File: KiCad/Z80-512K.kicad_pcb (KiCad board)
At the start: 2 copper layers, 99.1 x 49.9 mm, 32 parts, among them J1 VBAT, J2 JTAG, J3 RC2014_BUS, J4 RC2014_EXT, U1 Z84C00, U2 SST39SF040, U3 AS6C4008, U4 ATF1504AS, U5 ADM693A, X1 7.3728MHz

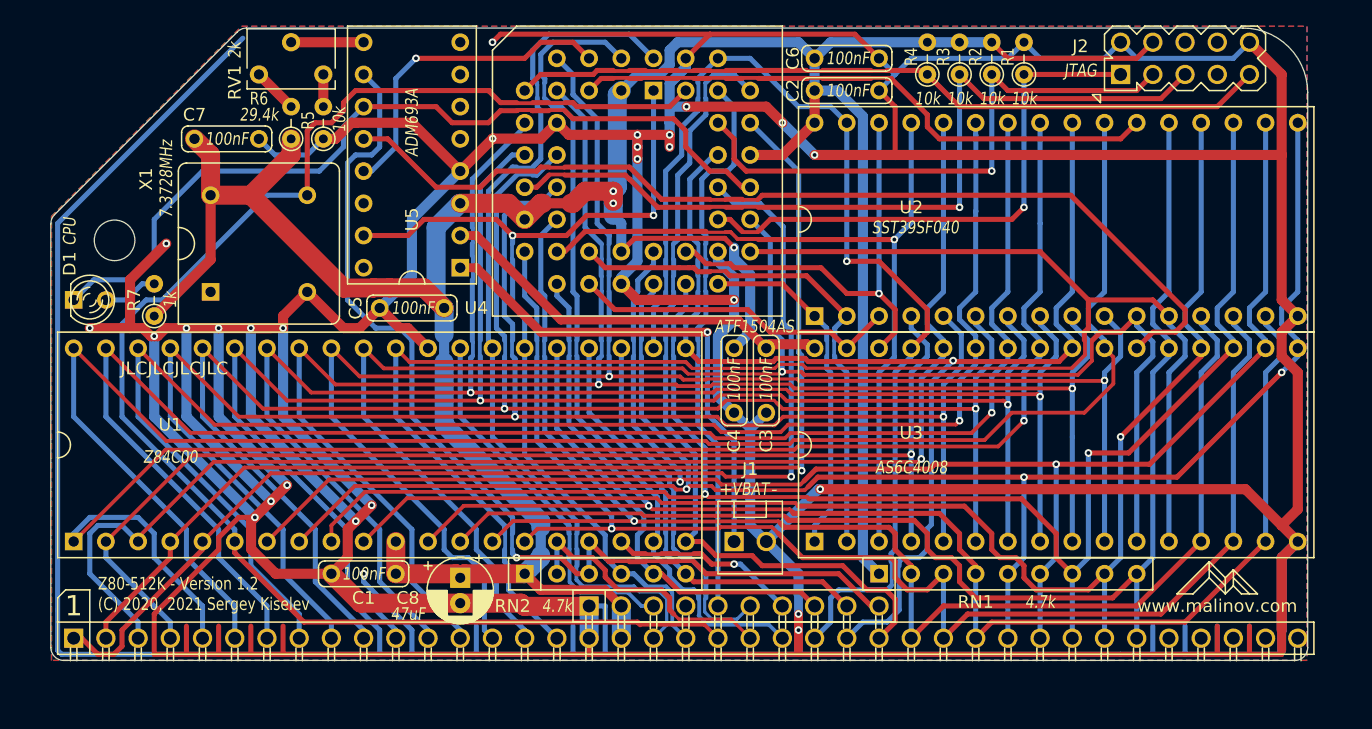
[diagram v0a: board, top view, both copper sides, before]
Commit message: Update files for V2.0
Signed-off-by: Sergey Kiselev <skiselev@gmail.com>
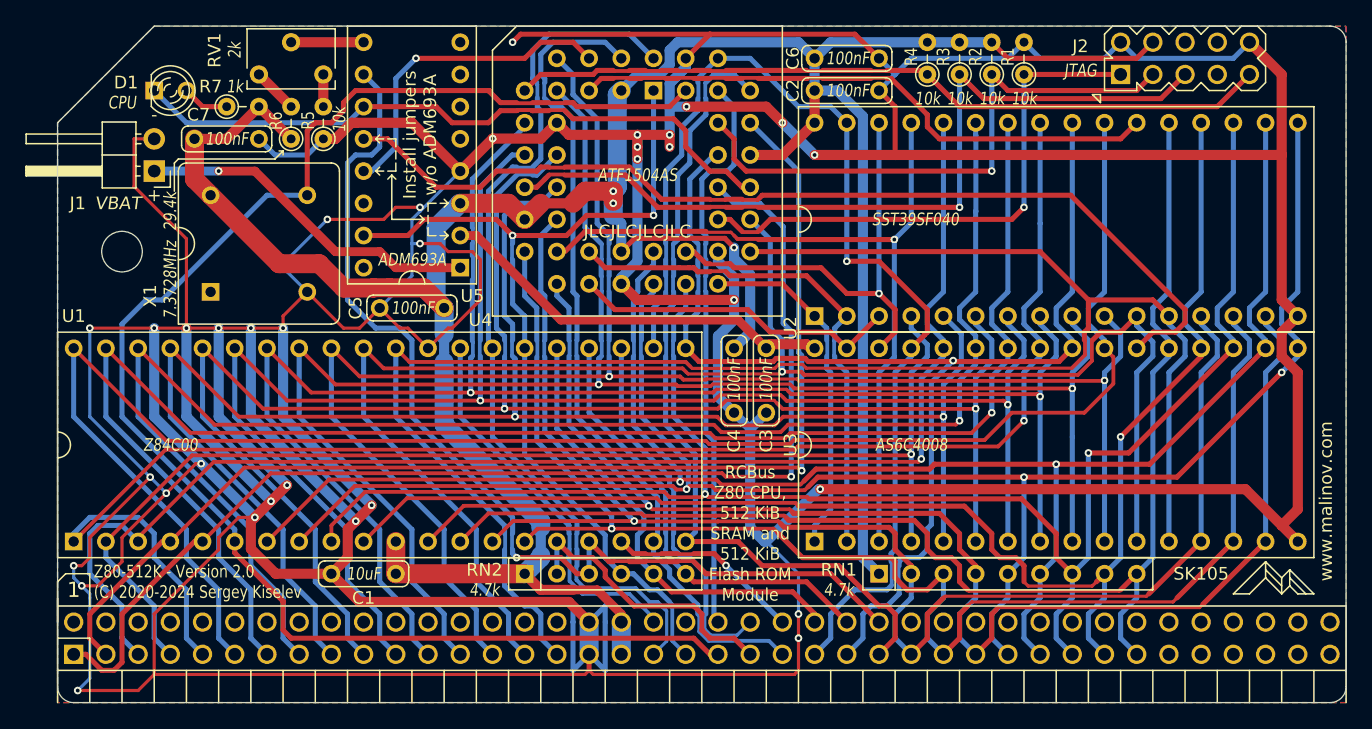
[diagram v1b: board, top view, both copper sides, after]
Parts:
- removed C8: 47uF, Capacitor_THT:CP_Radial_D5.0mm_P2.00mm
- removed J4: RC2014_EXT, My_Components:Conn_Pin_Header_10x1_2.54mm_Right_Angle
- C1: value 100nF -> 10uF
- J1: footprint My_Components:Conn_Friction_Lock_2P_2.54mm -> Connector_PinHeader_2.54mm:PinHeader_1x02_P2.54mm_Horizontal
- J3: value RC2014_BUS -> RCBus-80; footprint My_Components:Conn_Pin_Header_39x1_2.54mm_Right_Angle -> My_Components:Conn_Pin_Header_40x2_2.54mm_Right_Angle_RCBus80
- moved J1 55.3 mm to (133.3, 90.2), turned to 180 degrees
- moved D1 17.7 mm to (134.6, 83.8)
- moved R7 17.5 mm to (139.1, 85.1), turned to 0 degrees
- moved J3 1.27 mm to (175.3, 128.3)
- moved H1 1.06 mm to (130.8, 96.5)
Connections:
- net /~INT renamed /~{INT}
- net /~IORQ renamed /~{IORQ}
- net /~M1 renamed /~{M1}
- net /~MREQ renamed /~{MREQ}
- net /~RAM_CS renamed /~{RAM_CS}
- net /~RAM_CSI renamed /~{RAM_CSI}
- net /~RD renamed /~{RD}
- net /~RESET renamed /~{RESET}
- net /~ROM_CS renamed /~{ROM_CS}
- net /~WR renamed /~{WR}
- J2 pad 6: Net-(J2-Pad6) -> unconnected-(J2-Pad6)
- J2 pad 7: Net-(J2-Pad7) -> unconnected-(J2-Pad7)
- J2 pad 8: Net-(J2-Pad8) -> unconnected-(J2-Pad8)
- J3 pad 35: /TXDA -> unconnected-(J3-Pad35)
- J3 pad 36: /RXDA -> unconnected-(J3-Pad36)
- J3 pad 37: /USR1 -> unconnected-(J3-Pad37)
- J3 pad 38: /USR2 -> unconnected-(J3-Pad38)
- J3 pad 39: /USR3 -> unconnected-(J3-Pad39)
- R7 pad 1: VCC -> Net-(D1-Pad2)
- R7 pad 2: Net-(D1-Pad2) -> VCC
- RN2 pad 3: /~NMI -> /~{NMI}
- RN2 pad 5: /~BUSREQ -> /~{BUSREQ}
- RN2 pad 6: /~WAIT -> /~{WAIT}
- U1 pad 17: /~NMI -> /~{NMI}
- U1 pad 18: /~HALT -> /~{HALT}
- U1 pad 23: /~BUSACK -> /~{BUSACK}
- U1 pad 24: /~WAIT -> /~{WAIT}
- U1 pad 25: /~BUSREQ -> /~{BUSREQ}
- U1 pad 28: /~RFSH -> /~{RFSH}
- U5 pad 10: /~NMI -> /~{NMI}
- U5 pad 14: Net-(U5-Pad14) -> unconnected-(U5-Pad14)
- U5 pad 16: Net-(U5-Pad16) -> unconnected-(U5-Pad16)
- U5 pad 5: Net-(U5-Pad5) -> unconnected-(U5-Pad5)
- U5 pad 6: Net-(U5-Pad6) -> unconnected-(U5-Pad6)
- U5 pad 7: Net-(U5-Pad7) -> unconnected-(U5-Pad7)
- U5 pad 8: Net-(U5-Pad8) -> unconnected-(U5-Pad8)
- X1 pad 1: Net-(X1-Pad1) -> unconnected-(X1-Pad1)
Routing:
- net GND: track 842.0 -> 694.4 mm, vias 27 -> 34
- net /~{NMI}: track 0.00 -> 81.5 mm, vias 0 -> 1
- net /~NMI: track 81.0 -> 0.00 mm, vias 1 -> 0
- net /~{BUSREQ}: track 0.00 -> 36.0 mm
- net /~{WAIT}: track 0.00 -> 35.3 mm
- net /~BUSREQ: track 35.1 -> 0.00 mm
- net /~WAIT: track 34.8 -> 0.00 mm
- net /~{RFSH}: track 0.00 -> 30.1 mm
- net /~{BUSACK}: track 0.00 -> 29.5 mm
- net /~RFSH: track 29.4 -> 0.00 mm
- net /~BUSACK: track 28.2 -> 0.00 mm
- net VCC: track 258.5 -> 240.1 mm
- net /~{HALT}: track 0.00 -> 15.4 mm, vias 0 -> 1
- net /~HALT: track 14.9 -> 0.00 mm, vias 1 -> 0
- net /WDOG: track 71.5 -> 57.8 mm
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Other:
- board size 99.1 x 49.9 mm -> 101.6 x 53.3 mm
- net class Default removed
- net class Power removed
- board text added: "Install jumpers w/o ADM693A"
- board text added: "RCBus Z80 CPU, 512 KiB SRAM and 512 KiB Flash ROM Module"
- board text added: "SK105"
- board text added: "U5, C5, R5, R6, RV1 and J1 are optional - required for on-board CPU supervisor and battery-backed SRAM Install wire jumpers as indicated if not using this feature Connect 3V battery to J1 for battery-backed SRAM Place a jumper over J1 if battery backup is not required"
- board text added: "Z80-512K - Version 2.0 (C) 2020-2024 Sergey Kiselev"
- board text added: "Z80-512K - Version 2.0 Copyright (C) 2020 - 2024 Sergey Kiselev"
- board text removed: "1"
- board text removed: "A0"
- board text removed: "A1"
- board text removed: "A10"
- board text removed: "A11"
- board text removed: "A12"
- board text removed: "A13"
- board text removed: "A14"
- board text removed: "A15"
- board text removed: "A2"
- board text removed: "A3"
- board text removed: "A4"
- board text removed: "A5"
- board text removed: "A6"
- board text removed: "A7"
- board text removed: "A8"
- board text removed: "A9"
- board text removed: "Connect 3V battery to J1 for battery-backed SRAM Place a jumper over J1 if battery backup is not required"
- board text removed: "D0"
- board text removed: "D1"
- board text removed: "D2"
- board text removed: "D3"
- board text removed: "D4"
- board text removed: "D5"
- board text removed: "D6"
- board text removed: "D7"
- board text removed: "M1"
- board text removed: "RXDA"
- board text removed: "TXDA"
- board text removed: "USR1"
- board text removed: "USR2"
- board text removed: "USR3"
- board text removed: "Z80-512K - Version 1.2 (C) 2020, 2021 Sergey Kiselev"
- board text removed: "Z80-512K - Version 1.2 Copyright (C) 2020, 2021 Sergey Kiselev"
- board text removed: "~BACK"
- board text removed: "~BREQ"
- board text removed: "~CLK1"
- board text removed: "~CLK2"
- board text removed: "~HALT"
- board text removed: "~INT"
- board text removed: "~IORQ"
- board text removed: "~MREQ"
- board text removed: "~NMI"
- board text removed: "~RD"
- board text removed: "~RESET"
- board text removed: "~RFSH"
- board text removed: "~WAIT"
- board text removed: "~WR"
